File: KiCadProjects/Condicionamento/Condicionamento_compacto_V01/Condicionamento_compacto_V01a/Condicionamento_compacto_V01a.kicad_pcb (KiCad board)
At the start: 2 copper layers, 45 x 33 mm, 19 parts, among them J1 Entrada, J2 Canais, J3 Conn_01x03, J4 Conn_01x03, U1-Cond1 AD828AN

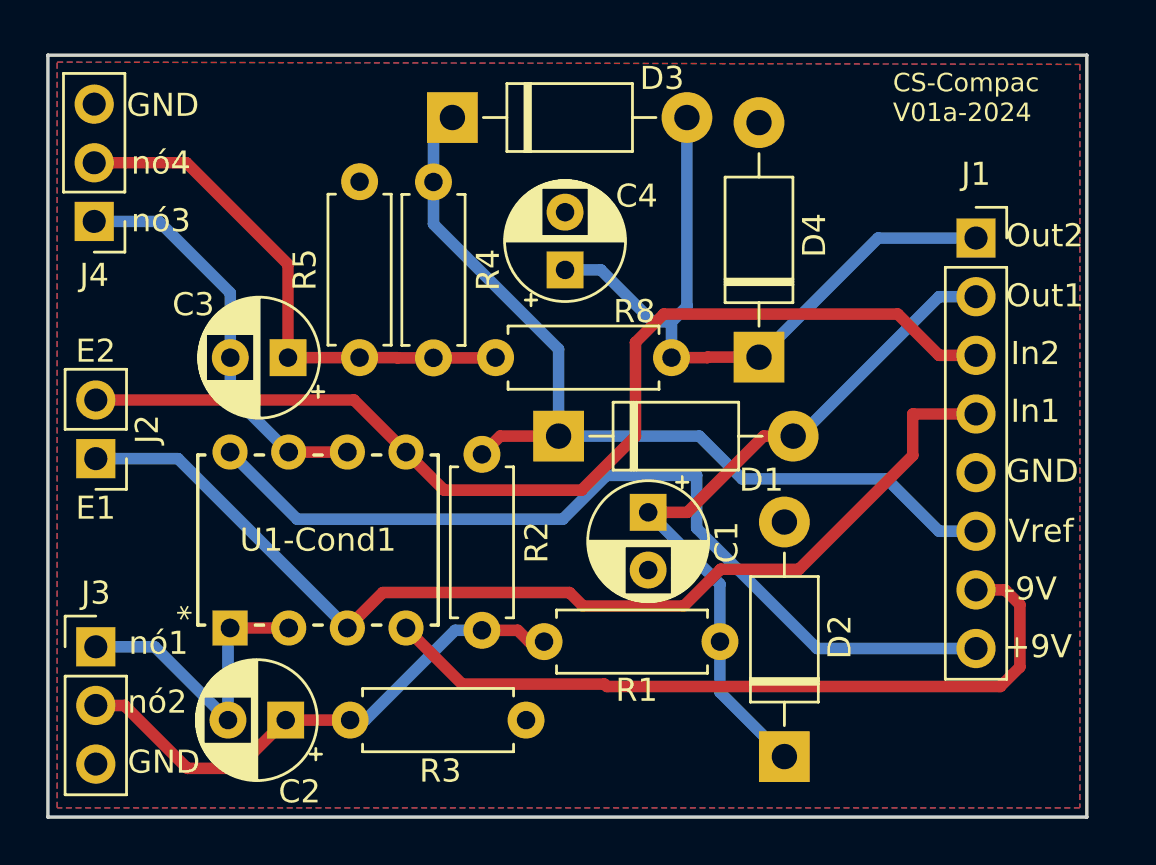
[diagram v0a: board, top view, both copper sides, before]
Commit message: lista de materiais
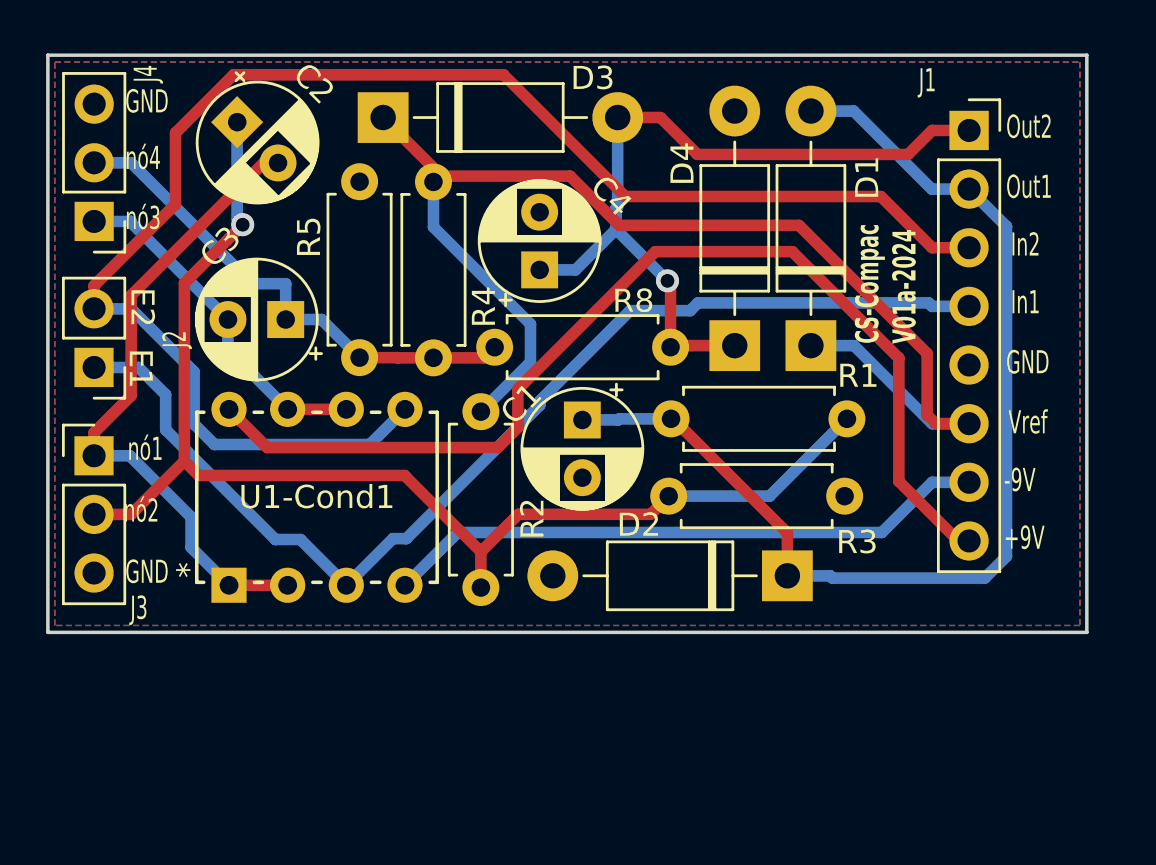
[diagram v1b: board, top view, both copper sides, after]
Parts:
- moved C2 26.0 mm to (130.3, 88.0), turned to -45 degrees
- moved R3 16.9 mm to (149.0, 104.2)
- moved R1 16.3 mm to (156.7, 100.8), turned to 180 degrees
- moved D1 11.6 mm to (155.2, 97.7), turned to 90 degrees
- moved J3 8.28 mm to (124.1, 102.5)
- moved D2 7.83 mm to (154.1, 107.7), turned to 180 degrees
- moved C1 4.91 mm to (145.2, 100.9)
- moved J1 4.67 mm to (162.0, 88.4)
- moved J2 3.95 mm to (124.1, 98.6)
- moved D3 3.00 mm to (136.6, 87.8)
- moved R2 1.85 mm to (140.9, 100.5)
- moved U1-Cond1 1.85 mm to (129.9, 108.1)
- moved C3 1.65 mm to (132.4, 96.5)
- moved D4 1.16 mm to (151.8, 97.7)
- moved C4 1.10 mm to (143.4, 94.4)
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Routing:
- net nó2: track 23.2 -> 55.0 mm, vias 0 -> 1
- net Canal_2: track 46.0 -> 65.5 mm
- net Out_1: track 31.1 -> 47.6 mm
- net nó1: track 13.6 -> 27.8 mm
- net Vref: track 39.8 -> 53.7 mm
- net +9V: track 38.7 -> 45.5 mm
- net -9V: track 32.9 -> 26.3 mm
- net nó3: track 17.7 -> 15.1 mm
- net Out_2: track 31.6 -> 34.1 mm, vias 0 -> 1
- net Canal_1: track 46.5 -> 47.9 mm
- net nó4: track 23.3 -> 21.9 mm
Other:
- board size 45 x 33 mm -> 45 x 25 mm
